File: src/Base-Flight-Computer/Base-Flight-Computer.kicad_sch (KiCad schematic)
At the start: 58 parts, among them J1 Jumper_NO, P1 1984659, P2 USB, P3 0530470610, P4 1984659, P5 B2B-PH-K-SLFSN_JST, Q1 QS5U17TR, Q2 2N7002W-7-F, Q3 2N7002W-7-F, Q4 QS5U17TR, Q5 2N7002W-7-F, Q6 2N7002W-7-F, U1 STM32G4A1KEU6, U2 BMP390, U3 LMS8117AMP-3.3_NOPB, U4 SST25VF040B-50-4I-S2AE-T, Y1 ECS-240-18-33-JGN-TR

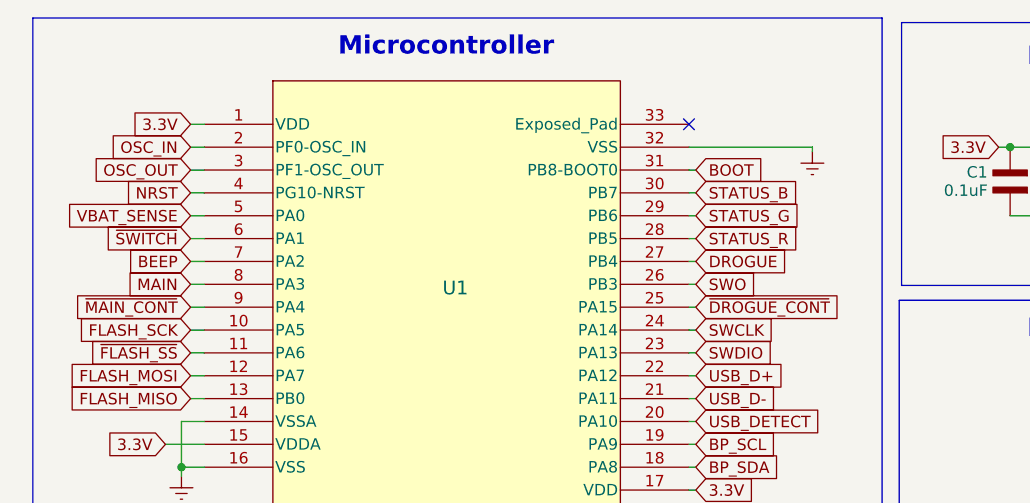
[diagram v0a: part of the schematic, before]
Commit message: created new project for preliminary hardware testing
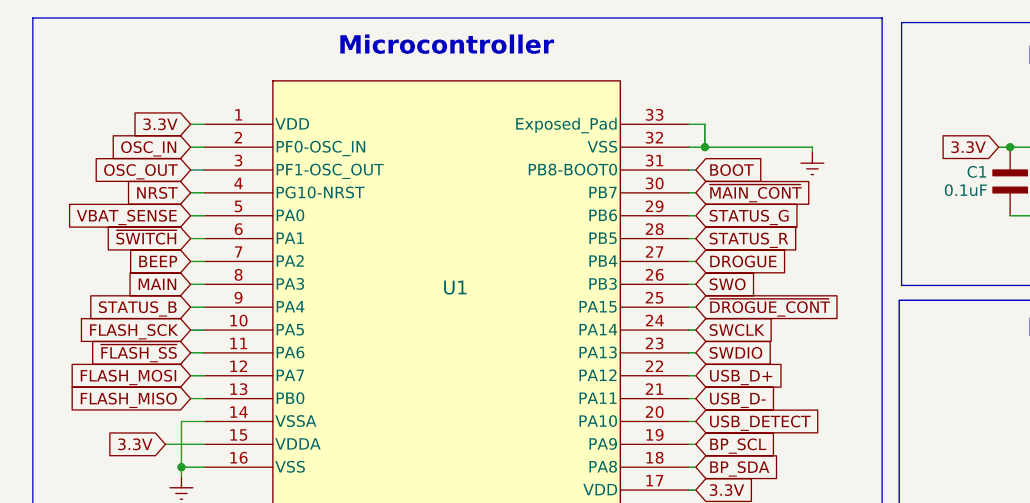
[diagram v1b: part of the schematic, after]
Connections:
- net Earth: now also U1.33 (Exposed_Pad)
- net STATUS_B: now also U1.9 (PA4); no longer U1.30 (PB7)
- net ~{MAIN_CONT}: now also U1.30 (PB7); no longer U1.9 (PA4)
- no-connect marks 3 -> 2
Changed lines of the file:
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@@
   (junction (at 144.399 174.117) (diameter 0) (color 0 0 0 0)
+  )
+  (junction (at 88.646 27.813) (diameter 0) (color 0 0 0 0)
   )
   (junction (at 40.132 100.203) (diameter 0) (color 0 0 0 0)
@@
   (no_connect (at 75.438 97.663))
   (no_connect (at 132.461 119.634))
-  (no_connect (at 86.868 25.273))
   (wire (pts (xy 86.868 53.213) (xy 87.63 53.213))
     (stroke (width 0) (type default))
@@
     (stroke (width 0) (type default))
   )
-  (wire (pts (xy 86.868 27.813) (xy 100.584 27.813))
+  (wire (pts (xy 86.868 27.813) (xy 88.646 27.813))
     (stroke (width 0) (type default))
   )
@@
     (stroke (width 0) (type default))
   )
+  (wire (pts (xy 86.868 25.273) (xy 88.646 25.273))
+    (stroke (width 0) (type default))
+  )
   (wire (pts (xy 86.868 30.353) (xy 87.63 30.353))
     (stroke (width 0) (type default))
@@
     (stroke (width 0) (type default))
   )
+  (wire (pts (xy 88.646 27.813) (xy 100.584 27.813))
+    (stroke (width 0) (type default))
+  )
   (wire (pts (xy 80.518 181.864) (xy 83.82 181.864))
     (stroke (width 0) (type default))
@@
     (stroke (width 0) (type default))
   )
+  (wire (pts (xy 31.496 45.593) (xy 33.02 45.593))
+    (stroke (width 0) (type default))
+  )
   (wire (pts (xy 216.789 153.797) (xy 216.789 154.813))
     (stroke (width 0) (type default))
@@
     (stroke (width 0) (type default))
   )
+  (wire (pts (xy 88.646 25.273) (xy 88.646 27.813))
+    (stroke (width 0) (type default))
+  )
   (wire (pts (xy 31.496 55.753) (xy 33.02 55.753))
     (stroke (width 0) (type default))
@@
   )
   (wire (pts (xy 46.228 129.794) (xy 46.228 125.603))
-    (stroke (width 0) (type default))
-  )
-  (wire (pts (xy 31.496 45.593) (xy 33.02 45.593))
     (stroke (width 0) (type default))
   )
@@
     )
   )
-  (global_label "~{MAIN_CONT}" (shape input) (at 31.496 45.593 180) (fields_autoplaced)
-    (effects (font (size 1.27 1.27)) (justify right))
-    (property "Intersheetrefs" "${INTERSHEET_REFS}" (at 18.7415 45.6724 0)
-      (effects (font (size 1.27 1.27)) (justify right) hide)
+  (global_label "~{MAIN_CONT}" (shape input) (at 87.63 32.893 0) (fields_autoplaced)
+    (effects (font (size 1.27 1.27)) (justify left))
+    (property "Intersheetrefs" "${INTERSHEET_REFS}" (at 100.3845 32.9724 0)
+      (effects (font (size 1.27 1.27)) (justify left) hide)
     )
   )
@@
     )
   )
-  (global_label "STATUS_B" (shape input) (at 87.63 32.893 0) (fields_autoplaced)
-    (effects (font (size 1.27 1.27)) (justify left))
-    (property "Intersheetrefs" "${INTERSHEET_REFS}" (at 99.0541 32.8136 0)
-      (effects (font (size 1.27 1.27)) (justify left) hide)
-    )
-  )
+  (global_label "STATUS_B" (shape input) (at 31.496 45.593 180) (fields_autoplaced)
+    (effects (font (size 1.27 1.27)) (justify right))
+    (property "Intersheetrefs" "${INTERSHEET_REFS}" (at 20.0719 45.5136 0)
+      (effects (font (size 1.27 1.27)) (justify right) hide)
+    )
+  )
